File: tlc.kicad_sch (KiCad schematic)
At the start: 13 parts, among them U5 TL074, U6 TL074, U7 TLC7528

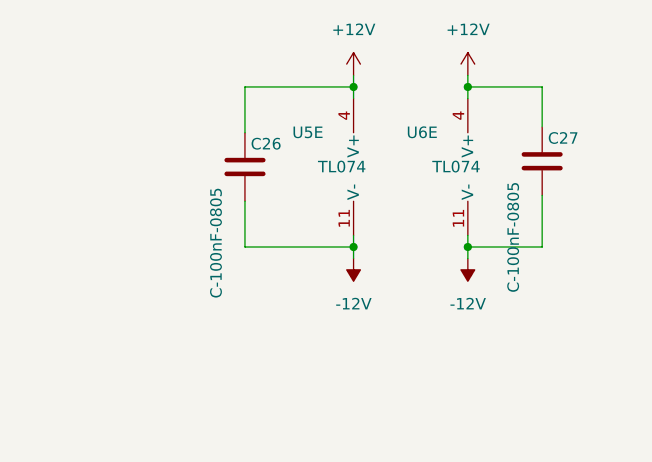
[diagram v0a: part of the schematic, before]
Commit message: wip
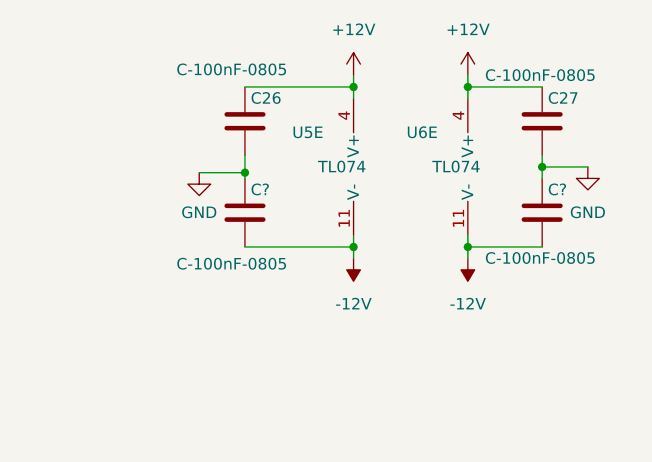
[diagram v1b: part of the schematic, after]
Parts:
- added C? (x2): C-100nF-0805, Capacitor_SMD:C_0805_2012Metric_Pad1.18x1.45mm_HandSolder, symbol eurorack:C-100nF-0805
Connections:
- net -12V: now also C?.2, C?.2; no longer C26.2, C27.2
- net GND: now also C26.2, C27.2, C?.1, C?.1
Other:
- moved on the sheet: C26, C27
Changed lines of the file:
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@@
   (junction (at 252.73 39.37) (diameter 0) (color 0 0 0 0)
   )
+  (junction (at 273.685 30.48) (diameter 0) (color 0 0 0 0)
+  )
   (junction (at 108.585 120.65) (diameter 0) (color 0 0 0 0)
   )
@@
   (junction (at 180.594 81.28) (diameter 0) (color 0 0 0 0)
   )
+  (junction (at 240.665 31.115) (diameter 0) (color 0 0 0 0)
+  )
   (wire (pts (xy 58.42 33.02) (xy 78.74 33.02))
     (stroke (width 0) (type default) (color 0 0 0 0))
@@
     (stroke (width 0) (type default) (color 0 0 0 0))
   )
+  (wire (pts (xy 235.585 31.115) (xy 240.665 31.115))
+    (stroke (width 0) (type default) (color 0 0 0 0))
+  )
   (wire (pts (xy 196.85 81.28) (xy 200.66 81.28))
     (stroke (width 0) (type default) (color 0 0 0 0))
@@
     (stroke (width 0) (type default) (color 0 0 0 0))
   )
-  (wire (pts (xy 273.685 21.59) (xy 273.685 26.035))
+  (wire (pts (xy 273.685 29.21) (xy 273.685 30.48))
     (stroke (width 0) (type default) (color 0 0 0 0))
   )
@@
     (stroke (width 0) (type default) (color 0 0 0 0))
   )
+  (wire (pts (xy 273.685 30.48) (xy 278.765 30.48))
+    (stroke (width 0) (type default) (color 0 0 0 0))
+  )
   (wire (pts (xy 200.66 86.36) (xy 203.2 86.36))
     (stroke (width 0) (type default) (color 0 0 0 0))
@@
     (stroke (width 0) (type default) (color 0 0 0 0))
   )
-  (wire (pts (xy 240.665 34.29) (xy 240.665 39.37))
-    (stroke (width 0) (type default) (color 0 0 0 0))
-  )
   (wire (pts (xy 158.75 54.61) (xy 158.75 62.865))
     (stroke (width 0) (type default) (color 0 0 0 0))
   )
+  (wire (pts (xy 273.685 30.48) (xy 273.685 31.75))
+    (stroke (width 0) (type default) (color 0 0 0 0))
+  )
   (wire (pts (xy 75.565 105.41) (xy 75.565 108.585))
     (stroke (width 0) (type default) (color 0 0 0 0))
@@
     (stroke (width 0) (type default) (color 0 0 0 0))
   )
+  (wire (pts (xy 240.665 31.115) (xy 240.665 31.75))
+    (stroke (width 0) (type default) (color 0 0 0 0))
+  )
   (wire (pts (xy 228.6 132.08) (xy 243.84 132.08))
     (stroke (width 0) (type default) (color 0 0 0 0))
@@
     (stroke (width 0) (type default) (color 0 0 0 0))
   )
+  (wire (pts (xy 240.665 29.21) (xy 240.665 31.115))
+    (stroke (width 0) (type default) (color 0 0 0 0))
+  )
   (wire (pts (xy 200.66 93.98) (xy 207.01 93.98))
     (stroke (width 0) (type default) (color 0 0 0 0))
@@
     (stroke (width 0) (type default) (color 0 0 0 0))
   )
-  (wire (pts (xy 240.665 26.67) (xy 240.665 21.59))
-    (stroke (width 0) (type default) (color 0 0 0 0))
-  )
   (wire (pts (xy 154.94 96.52) (xy 154.94 110.49))
     (stroke (width 0) (type default) (color 0 0 0 0))
@@
   )
   (wire (pts (xy 223.52 93.98) (xy 223.52 101.6))
-    (stroke (width 0) (type default) (color 0 0 0 0))
-  )
-  (wire (pts (xy 273.685 33.655) (xy 273.685 39.37))
     (stroke (width 0) (type default) (color 0 0 0 0))
   )
@@
     (effects (font (size 1.27 1.27)) (justify right))
   )
-  (symbol (lib_id "eurorack:C-100nF-0805") (at 273.685 29.845 0) (unit 1)
-    (in_bom yes) (on_board yes)
-    (property "Reference" "C27" (id 0) (at 274.32 27.305 0)
-      (effects (font (size 1.27 1.27)) (justify left))
-    )
-    (property "Value" "C-100nF-0805" (id 1) (at 270.51 44.45 90)
-      (effects (font (size 1.27 1.27)) (justify left))
-    )
-    (property "Footprint" "Capacitor_SMD:C_0805_2012Metric_Pad1.18x1.45mm_HandSolder" (id 2) (at 274.6502 33.655 0)
-      (effects (font (size 1.27 1.27)) hide)
-    )
-    (property "Datasheet" "https://secure.reichelt.com/at/en/smd-multilayer-ceramic-capacitor-100-n-10--x7r-g0805-100n-p31879.html?&nbc=1" (id 3) (at 273.685 29.845 0)
+  (symbol (lib_id "eurorack:C-100nF-0805") (at 273.685 25.4 0) (unit 1)
+    (in_bom yes) (on_board yes)
+    (property "Reference" "C27" (id 0) (at 274.32 22.86 0)
+      (effects (font (size 1.27 1.27)) (justify left))
+    )
+    (property "Value" "C-100nF-0805" (id 1) (at 267.335 20.32 0)
+      (effects (font (size 1.27 1.27)) (justify left))
+    )
+    (property "Footprint" "Capacitor_SMD:C_0805_2012Metric_Pad1.18x1.45mm_HandSolder" (id 2) (at 274.6502 29.21 0)
+      (effects (font (size 1.27 1.27)) hide)
+    )
+    (property "Datasheet" "https://secure.reichelt.com/at/en/smd-multilayer-ceramic-capacitor-100-n-10--x7r-g0805-100n-p31879.html?&nbc=1" (id 3) (at 273.685 25.4 0)
+      (effects (font (size 1.27 1.27)) hide)
+    )
+    (pin "1")
+    (pin "2")
+  )
+  (symbol (lib_id "eurorack:C-100nF-0805") (at 273.685 35.56 0) (unit 1)
+    (in_bom yes) (on_board yes)
+    (property "Reference" "C?" (id 0) (at 274.32 33.02 0)
+      (effects (font (size 1.27 1.27)) (justify left))
+    )
+    (property "Value" "C-100nF-0805" (id 1) (at 267.335 40.64 0)
+      (effects (font (size 1.27 1.27)) (justify left))
+    )
+    (property "Footprint" "Capacitor_SMD:C_0805_2012Metric_Pad1.18x1.45mm_HandSolder" (id 2) (at 274.6502 39.37 0)
+      (effects (font (size 1.27 1.27)) hide)
+    )
+    (property "Datasheet" "https://secure.reichelt.com/at/en/smd-multilayer-ceramic-capacitor-100-n-10--x7r-g0805-100n-p31879.html?&nbc=1" (id 3) (at 273.685 35.56 0)
       (effects (font (size 1.27 1.27)) hide)
     )
@@
     (pin "9")
   )
+  (symbol (lib_id "power:GND") (at 235.585 31.115 0) (unit 1)
+    (in_bom yes) (on_board yes) (fields_autoplaced)
+    (property "Reference" "#PWR?" (id 0) (at 235.585 37.465 0)
+      (effects (font (size 1.27 1.27)) hide)
+    )
+    (property "Value" "GND" (id 1) (at 235.585 35.56 0))
+    (property "Footprint" "" (id 2) (at 235.585 31.115 0)
+      (effects (font (size 1.27 1.27)) hide)
+    )
+    (property "Datasheet" "" (id 3) (at 235.585 31.115 0)
+      (effects (font (size 1.27 1.27)) hide)
+    )
+    (pin "1")
+  )
   (symbol (lib_id "eurorack:R-10k-1206") (at 210.82 93.98 90) (unit 1)
     (in_bom yes) (on_board yes)
@@
     (pin "4")
   )
-  (symbol (lib_id "eurorack:C-100nF-0805") (at 240.665 30.48 0) (unit 1)
-    (in_bom yes) (on_board yes)
-    (property "Reference" "C26" (id 0) (at 241.3 27.94 0)
-      (effects (font (size 1.27 1.27)) (justify left))
-    )
-    (property "Value" "C-100nF-0805" (id 1) (at 237.49 45.085 90)
-      (effects (font (size 1.27 1.27)) (justify left))
-    )
-    (property "Footprint" "Capacitor_SMD:C_0805_2012Metric_Pad1.18x1.45mm_HandSolder" (id 2) (at 241.6302 34.29 0)
-      (effects (font (size 1.27 1.27)) hide)
-    )
-    (property "Datasheet" "https://secure.reichelt.com/at/en/smd-multilayer-ceramic-capacitor-100-n-10--x7r-g0805-100n-p31879.html?&nbc=1" (id 3) (at 240.665 30.48 0)
+  (symbol (lib_id "eurorack:C-100nF-0805") (at 240.665 25.4 0) (unit 1)
+    (in_bom yes) (on_board yes)
+    (property "Reference" "C26" (id 0) (at 241.3 22.86 0)
+      (effects (font (size 1.27 1.27)) (justify left))
+    )
+    (property "Value" "C-100nF-0805" (id 1) (at 233.045 19.685 0)
+      (effects (font (size 1.27 1.27)) (justify left))
+    )
+    (property "Footprint" "Capacitor_SMD:C_0805_2012Metric_Pad1.18x1.45mm_HandSolder" (id 2) (at 241.6302 29.21 0)
+      (effects (font (size 1.27 1.27)) hide)
+    )
+    (property "Datasheet" "https://secure.reichelt.com/at/en/smd-multilayer-ceramic-capacitor-100-n-10--x7r-g0805-100n-p31879.html?&nbc=1" (id 3) (at 240.665 25.4 0)
       (effects (font (size 1.27 1.27)) hide)
     )
@@
     (pin "4")
   )
+  (symbol (lib_id "eurorack:C-100nF-0805") (at 240.665 35.56 0) (unit 1)
+    (in_bom yes) (on_board yes)
+    (property "Reference" "C?" (id 0) (at 241.3 33.02 0)
+      (effects (font (size 1.27 1.27)) (justify left))
+    )
+    (property "Value" "C-100nF-0805" (id 1) (at 233.045 41.275 0)
+      (effects (font (size 1.27 1.27)) (justify left))
+    )
+    (property "Footprint" "Capacitor_SMD:C_0805_2012Metric_Pad1.18x1.45mm_HandSolder" (id 2) (at 241.6302 39.37 0)
+      (effects (font (size 1.27 1.27)) hide)
+    )
+    (property "Datasheet" "https://secure.reichelt.com/at/en/smd-multilayer-ceramic-capacitor-100-n-10--x7r-g0805-100n-p31879.html?&nbc=1" (id 3) (at 240.665 35.56 0)
+      (effects (font (size 1.27 1.27)) hide)
+    )
+    (pin "1")
+    (pin "2")
+  )
   (symbol (lib_id "power:GND") (at 75.565 108.585 0) (unit 1)
     (in_bom yes) (on_board yes) (fields_autoplaced)
@@
       (effects (font (size 1.27 1.27)) hide)
     )
+    (pin "1")
+  )
+  (symbol (lib_id "power:GND") (at 278.765 30.48 0) (unit 1)
+    (in_bom yes) (on_board yes) (fields_autoplaced)
+    (property "Reference" "#PWR?" (id 0) (at 278.765 36.83 0)
+      (effects (font (size 1.27 1.27)) hide)
+    )
+    (property "Value" "GND" (id 1) (at 278.765 35.56 0))
+    (property "Footprint" "" (id 2) (at 278.765 30.48 0)
+      (effects (font (size 1.27 1.27)) hide)
+    )
+    (property "Datasheet" "" (id 3) (at 278.765 30.48 0)
+      (effects (font (size 1.27 1.27)) hide)
+    )
